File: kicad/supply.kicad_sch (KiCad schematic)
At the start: 26 parts, among them J1 Battery Connector, P1 USB_C_Plug_USB2.0, U2 CP2102N-Axx-xQFN20, U3 MCP73831-2-OT, U4 BCM857BS, U5 ME6211H33M5G

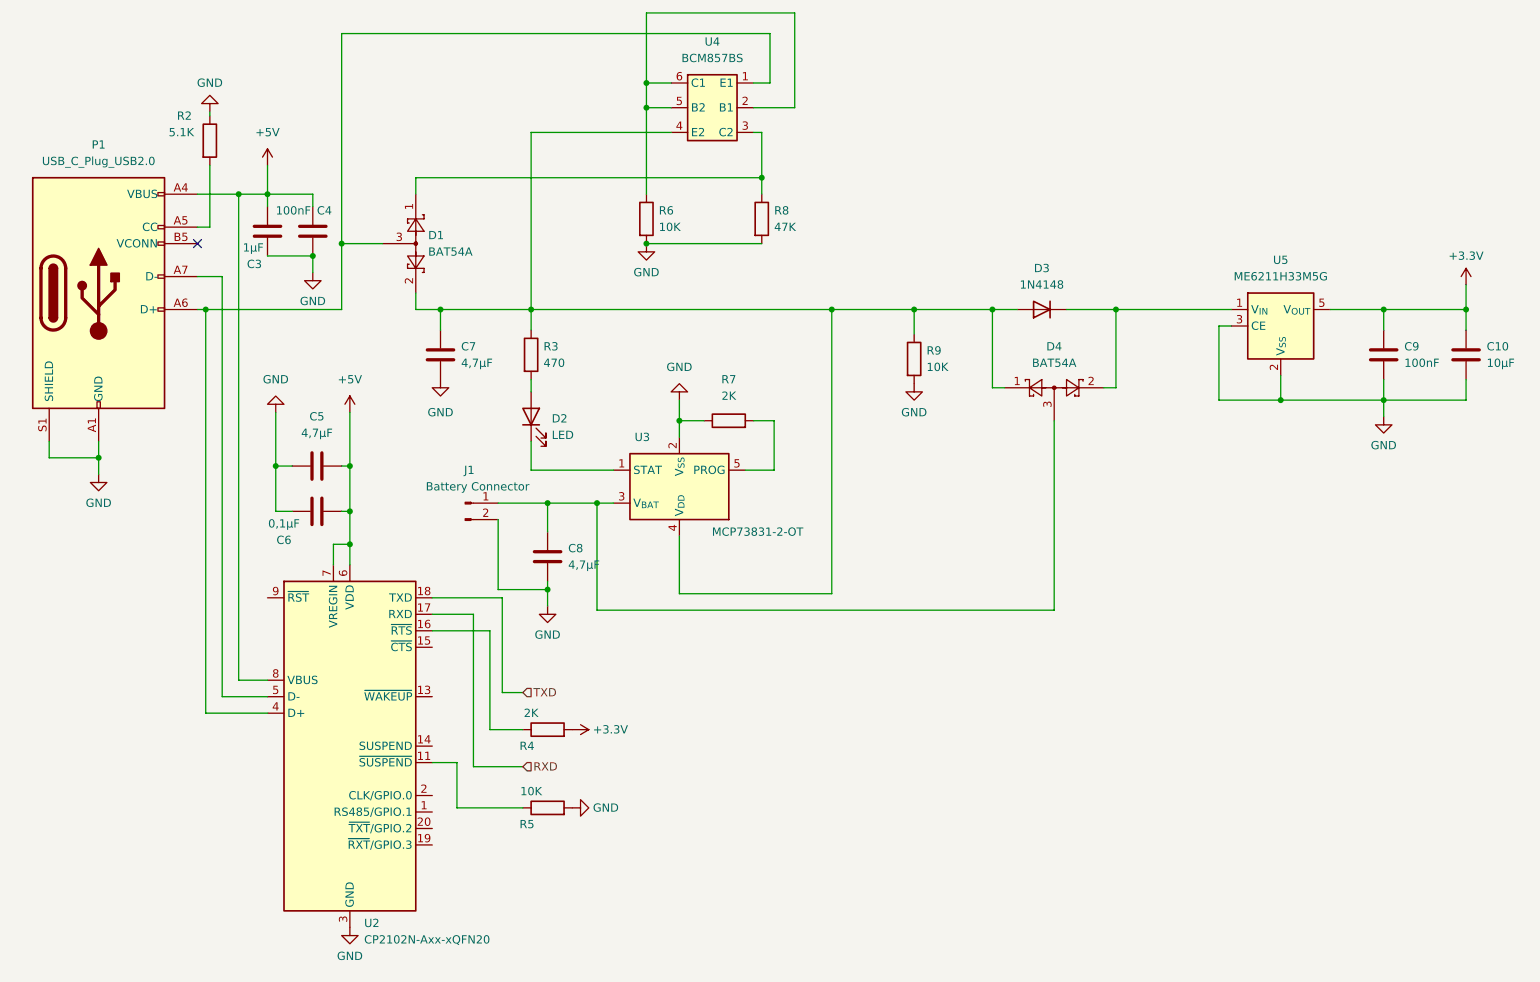
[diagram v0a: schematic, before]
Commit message: init
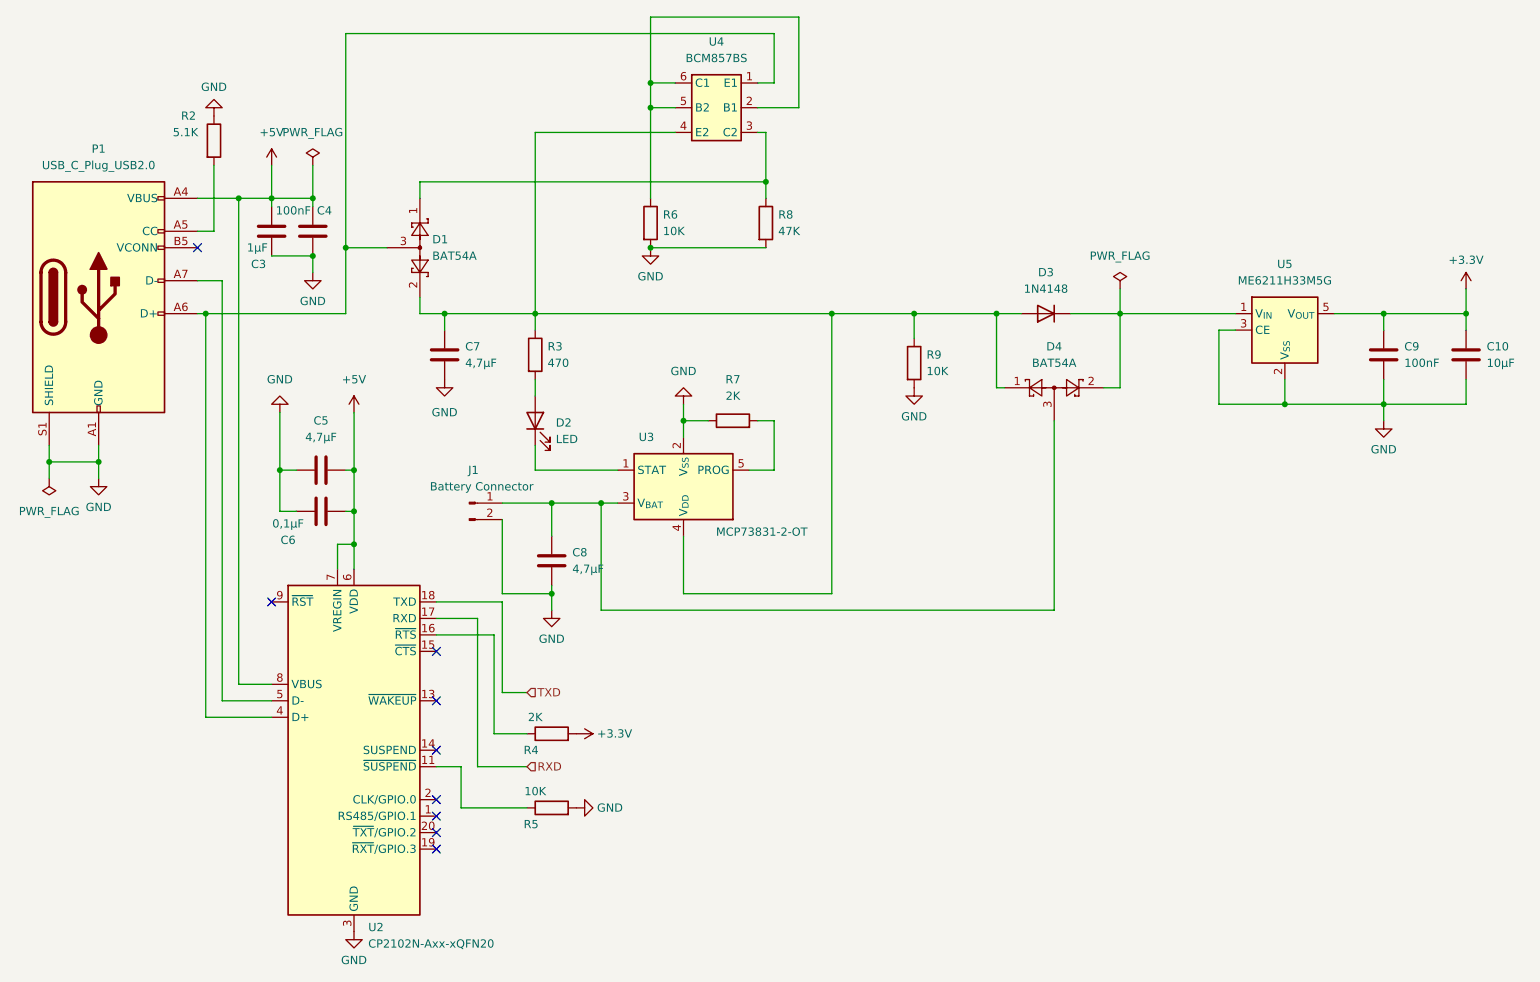
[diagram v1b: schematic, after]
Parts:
- R2: footprint Resistor_SMD:R_2816_7142Metric -> Resistor_SMD:R_0805_2012Metric; LCSC (none) -> C57864
- R3: footprint Resistor_SMD:R_2816_7142Metric -> Resistor_SMD:R_1206_3216Metric; LCSC (none) -> C4502
- R4, R5, R6, R7, R8, R9: footprint Resistor_SMD:R_2816_7142Metric -> Resistor_SMD:R_1206_3216Metric
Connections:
- no-connect marks 1 -> 9
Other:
- moved on the sheet: C3, C5, C6, C7, C8, D1, D2, D3, J1, P1, R2, R3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
